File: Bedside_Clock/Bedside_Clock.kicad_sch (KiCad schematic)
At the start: 45 parts, among them J1 USBC_USB2.0, SW1 COLOR, SW2 MODE, SW3 BOOT, SW4 RESET, U1 ESP32-C3-MINI-1, U2 USBLC6-2SC6, U3 VCNL4040M3OE, U4 SN74LVC2T45DCTR, U5 MCP1825S

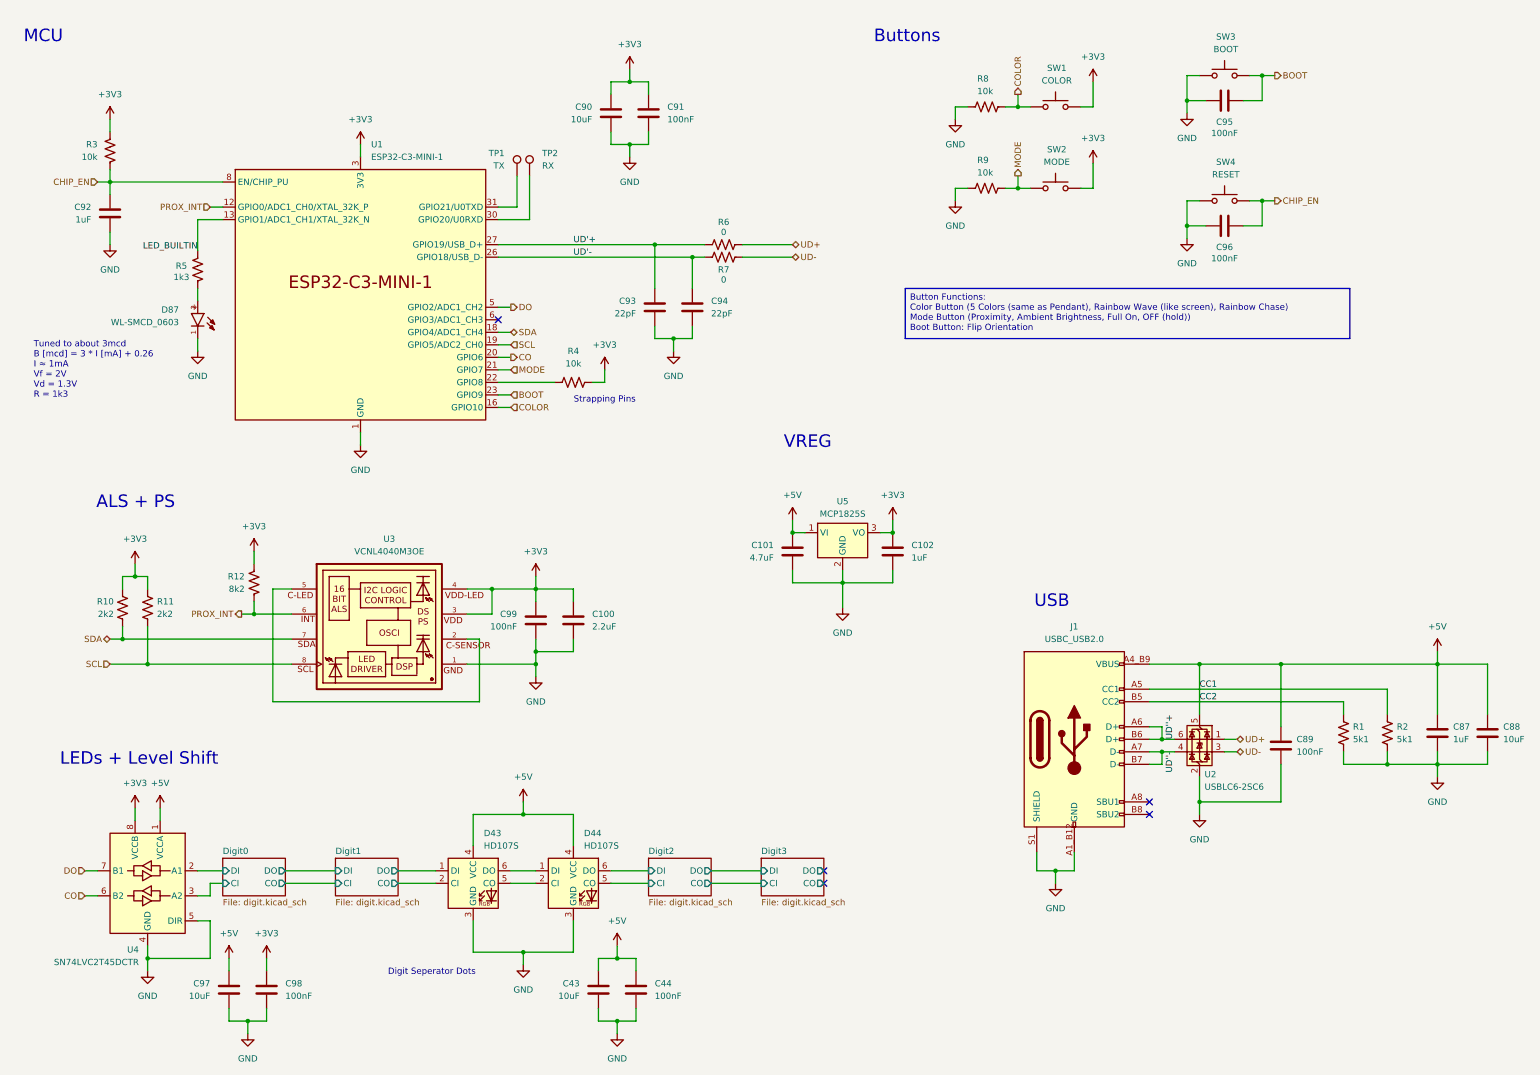
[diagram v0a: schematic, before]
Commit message: [Docs] Add Schematics and Renders Add Diodes, Switches, and Conns to BOM Need Resistors and Capacitors now
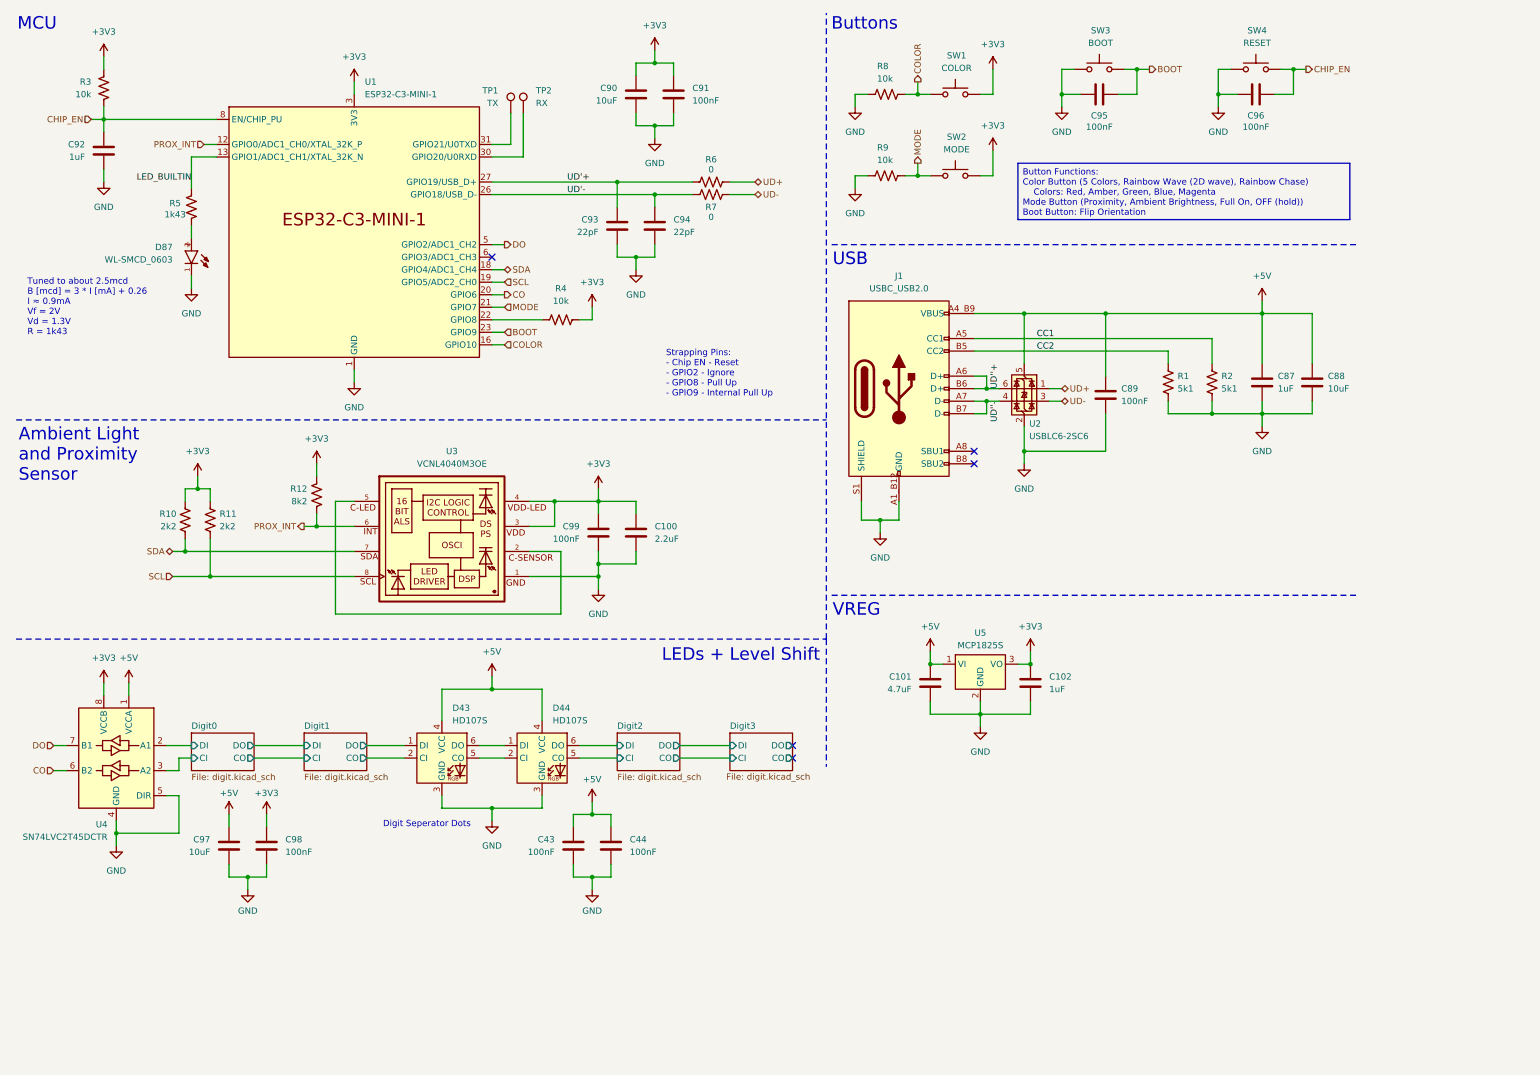
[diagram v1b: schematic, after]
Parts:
- C43: value 10uF -> 100nF
- R5: value 1k3 -> 1k43
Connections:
- net +5V: no longer J1.A5 (CC1), J1.B5 (CC2), R1.2, R2.2
- new net CC1: J1.A5 (CC1), R2.2
- new net CC2: J1.B5 (CC2), R1.2
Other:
- note added: "Ambient Light and Proximity Sensor"
- note added: "Strapping Pins: - Chip EN - Reset - GPIO2 - Ignore - GPIO8 - Pull Up - GPIO9 - Internal Pull Up"
- note added: "Tuned to about 2.5mcd B [mcd] = 3 * I [mA] + 0.26 I ≈ 0.9mA Vf = 2V Vd = 1.3V R = 1k43"
- note removed: "ALS + PS"
- note removed: "Strapping Pins"
- note removed: "Tuned to about 3mcd B [mcd] = 3 * I [mA] + 0.26 I ≈ 1mA Vf = 2V Vd = 1.3V R = 1k3"
- moved on the sheet: C100, C101, C102, C43, C44, C87, C88, C89, C90, C91, C92, C93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
